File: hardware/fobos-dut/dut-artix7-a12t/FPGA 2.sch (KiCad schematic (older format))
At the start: 1 part, among them U1 XC7A12T-CSG325

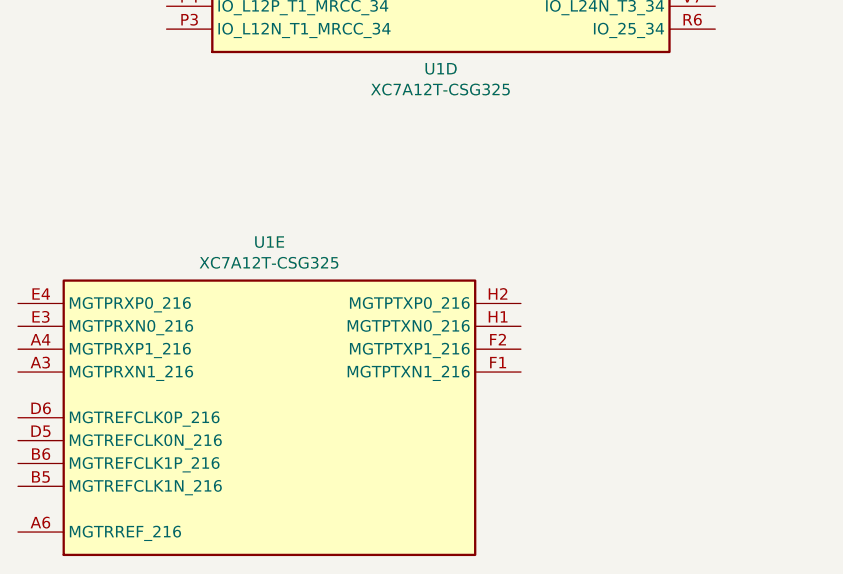
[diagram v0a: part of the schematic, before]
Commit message: Preliminary placement underway Made a copy of cerg 3d model within Artix 7 dut project to resolve nagging library path issue
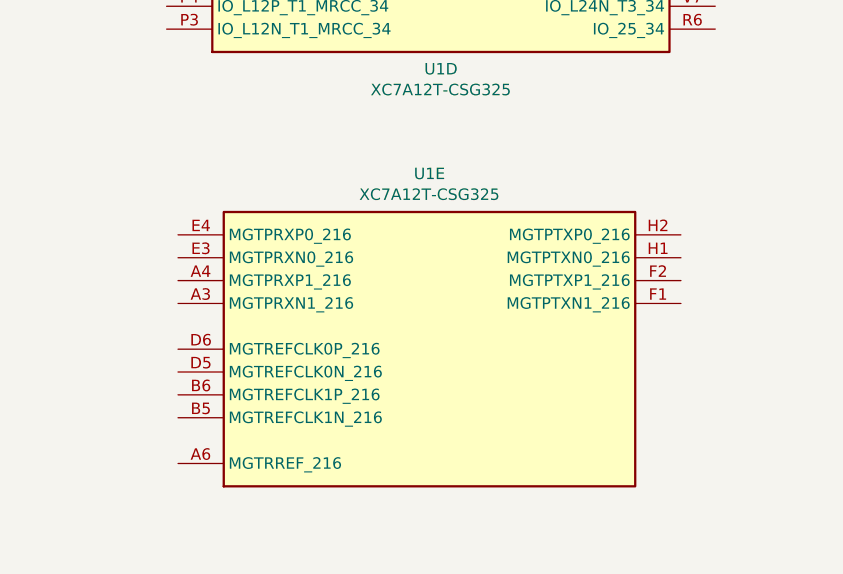
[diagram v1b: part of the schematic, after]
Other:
- moved on the sheet: U1E
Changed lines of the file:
@@
 L cerg:XC7A12T-CSG325 U?
 U 5 1 6008248E
-P 2850 6150
+P 3550 5850
 AR Path="/5F22D594/6008248E" Ref="U?"  Part="5"
 AR Path="/6004C151/6008248E" Ref="U1"  Part="5"
-F 0 "U1" H 2850 6917 50  0000 C CNN
-F 1 "XC7A12T-CSG325" H 2850 6826 50  0000 C CNN
-F 2 "Package_BGA:Xilinx_CSG325" H 2850 6150 50  0001 C CNN
-F 3 "https://www.xilinx.com/support/documentation/data_sheets/ds180_7Series_Overview.pdf" H 2850 6150 50  0001 C CNN
-	5    2850 6150
+F 0 "U1" H 3550 6617 50  0000 C CNN
+F 1 "XC7A12T-CSG325" H 3550 6526 50  0000 C CNN
+F 2 "Package_BGA:Xilinx_CSG325" H 3550 5850 50  0001 C CNN
+F 3 "https://www.xilinx.com/support/documentation/data_sheets/ds180_7Series_Overview.pdf" H 3550 5850 50  0001 C CNN
+	5    3550 5850
 	1    0    0    -1
 $EndComp
